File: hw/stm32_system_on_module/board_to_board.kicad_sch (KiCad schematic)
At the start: 2 parts, among them J2 DF40C-50DP-0.4V_51_, J3 DF40C-50DP-0.4V_51_

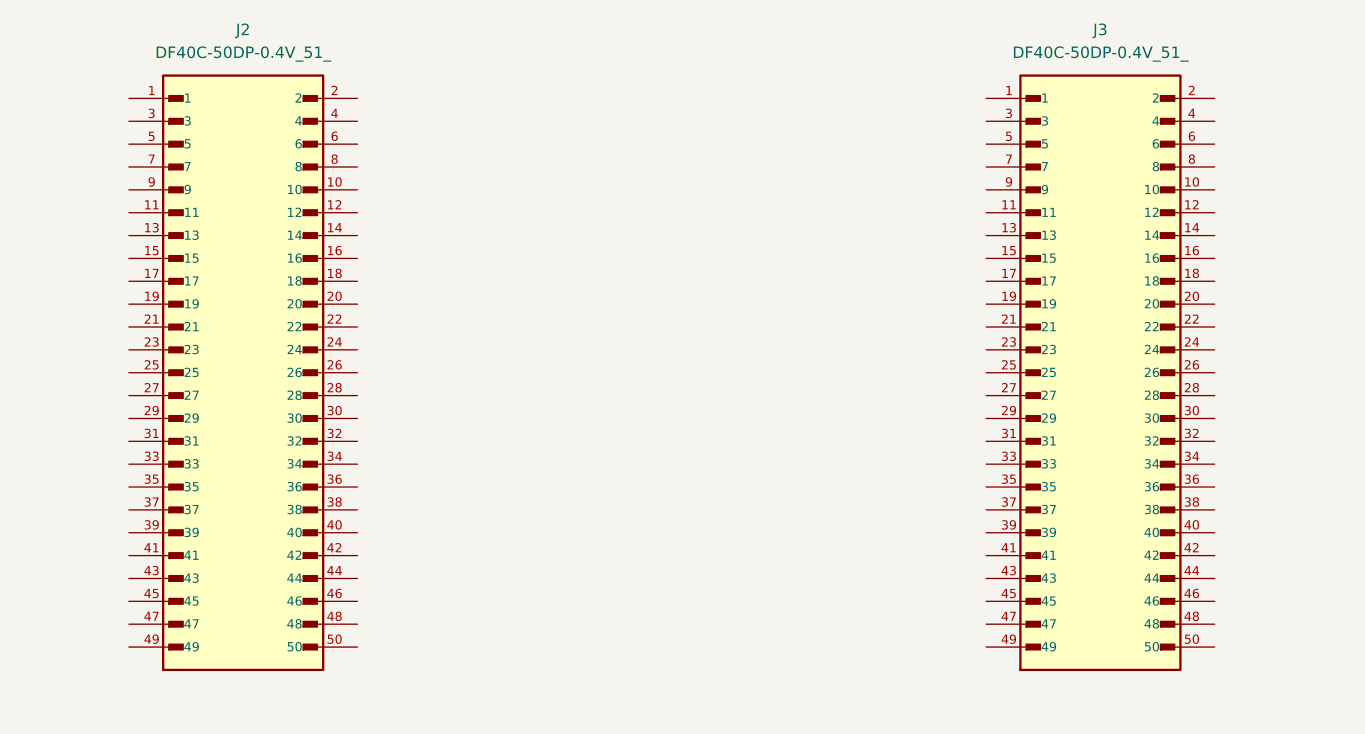
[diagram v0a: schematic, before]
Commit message: HW finished
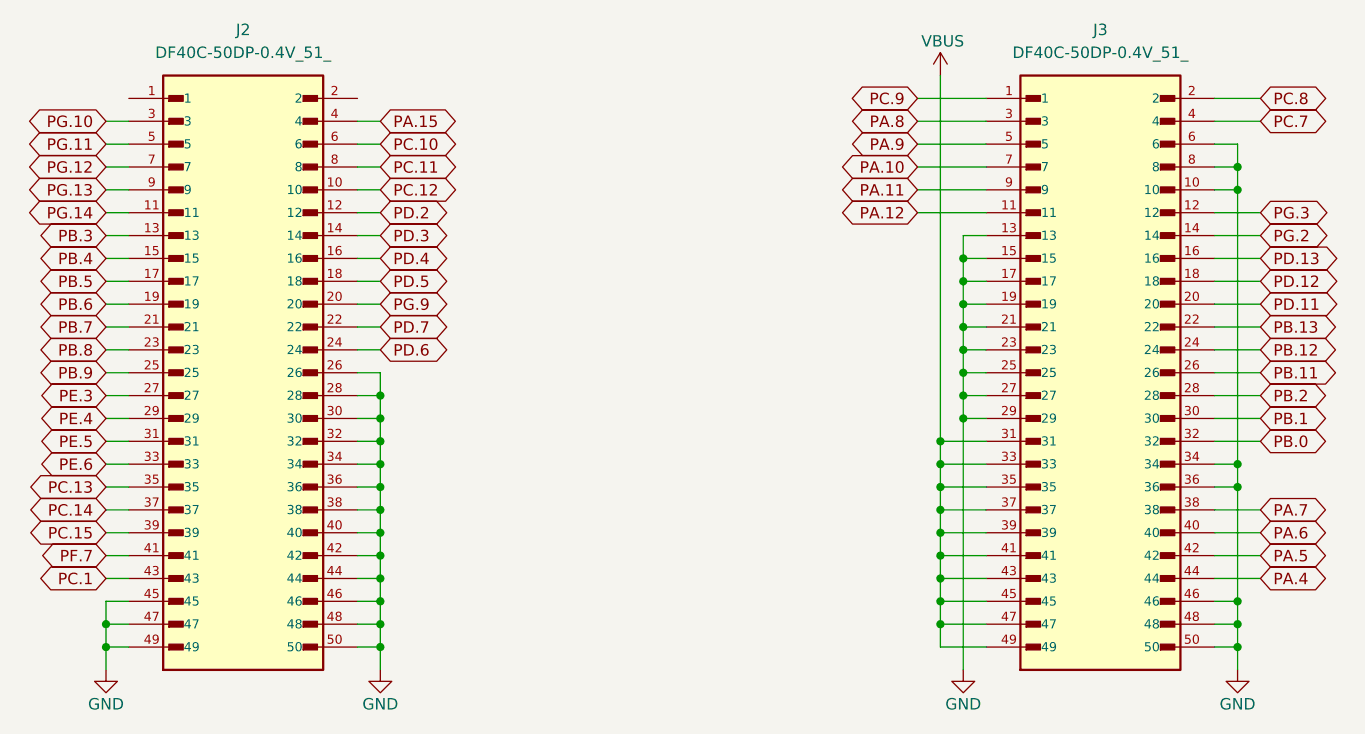
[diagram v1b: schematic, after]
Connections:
- net PC.9: now reaches J3.1
- net GND: now reaches J3.10
- net GND: now also J2.26, J2.28, J2.30, J2.32, J2.34, J2.36, J2.38, J2.40, J2.42, J2.44, J2.45, J2.46, J2.47, J2.48, J2.49, J2.50, J3.13, J3.15, J3.17, J3.19, J3.21, J3.23, J3.25, J3.27, J3.29, J3.34, J3.36, J3.46, J3.48, J3.50, J3.6, J3.8
- net PA.12: now reaches J3.11
- net PG.3: now reaches J3.12
- net PG.2: now reaches J3.14
- net PD.13: now reaches J3.16
- net PD.12: now reaches J3.18
- net PC.8: now reaches J3.2
- net PD.11: now reaches J3.20
- net PB.13: now reaches J3.22
- net PB.12: now reaches J3.24
- net PB.11: now reaches J3.26
- net PB.2: now reaches J3.28
- net PA.8: now reaches J3.3
- net PB.1: now reaches J3.30
- net VBUS: now reaches J3.31
- net VBUS: now also J3.33, J3.35, J3.37, J3.39, J3.41, J3.43, J3.45, J3.47, J3.49
- net PB.0: now reaches J3.32
- net PA.7: now reaches J3.38
- net PC.7: now reaches J3.4
- net PA.6: now reaches J3.40
- net PA.5: now reaches J3.42
- net PA.4: now reaches J3.44
- net PA.9: now reaches J3.5
- net PA.10: now reaches J3.7
- net PA.11: now reaches J3.9
- net PC.12: now reaches J2.10
- net PG.14: now reaches J2.11
- net PD.2: now reaches J2.12
- net PB.3: now reaches J2.13
- net PD.3: now reaches J2.14
- net PB.4: now reaches J2.15
- net PD.4: now reaches J2.16
- net PB.5: now reaches J2.17
- net PD.5: now reaches J2.18
- net PB.6: now reaches J2.19
- net PG.9: now reaches J2.20
- net PB.7: now reaches J2.21
- net PD.7: now reaches J2.22
- net PB.8: now reaches J2.23
- net PD.6: now reaches J2.24
- net PB.9: now reaches J2.25
- net PE.3: now reaches J2.27
- net PE.4: now reaches J2.29
- net PG.10: now reaches J2.3
- net PE.5: now reaches J2.31
- net PE.6: now reaches J2.33
- net PC.13: now reaches J2.35
- net PC.14: now reaches J2.37
- net PC.15: now reaches J2.39
- net PA.15: now reaches J2.4
- net PF.7: now reaches J2.41
- net PC.1: now reaches J2.43
- net PG.11: now reaches J2.5
- net PC.10: now reaches J2.6
- net PG.12: now reaches J2.7
- net PC.11: now reaches J2.8
- net PG.13: now reaches J2.9
